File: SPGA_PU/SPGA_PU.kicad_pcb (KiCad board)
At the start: 2 copper layers, 16 parts, among them Q3 NMOS

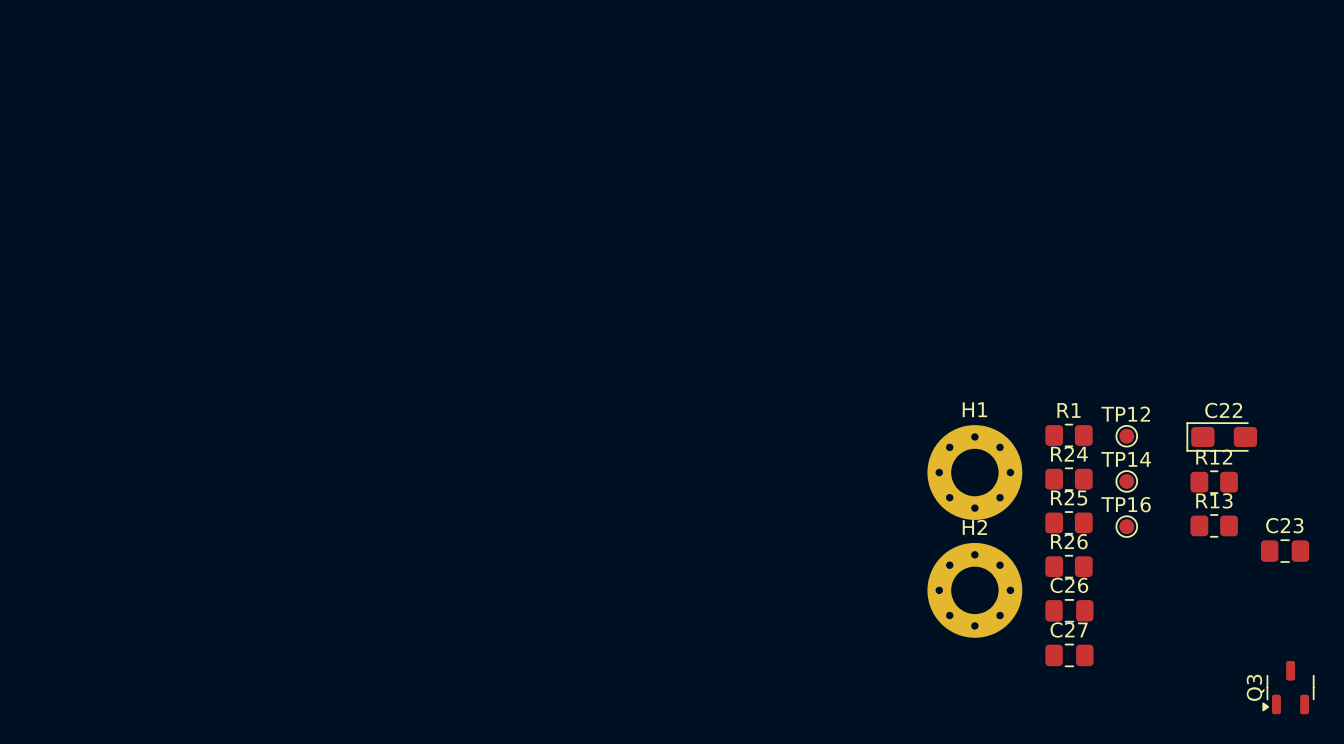
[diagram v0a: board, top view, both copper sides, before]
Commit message: I dunno
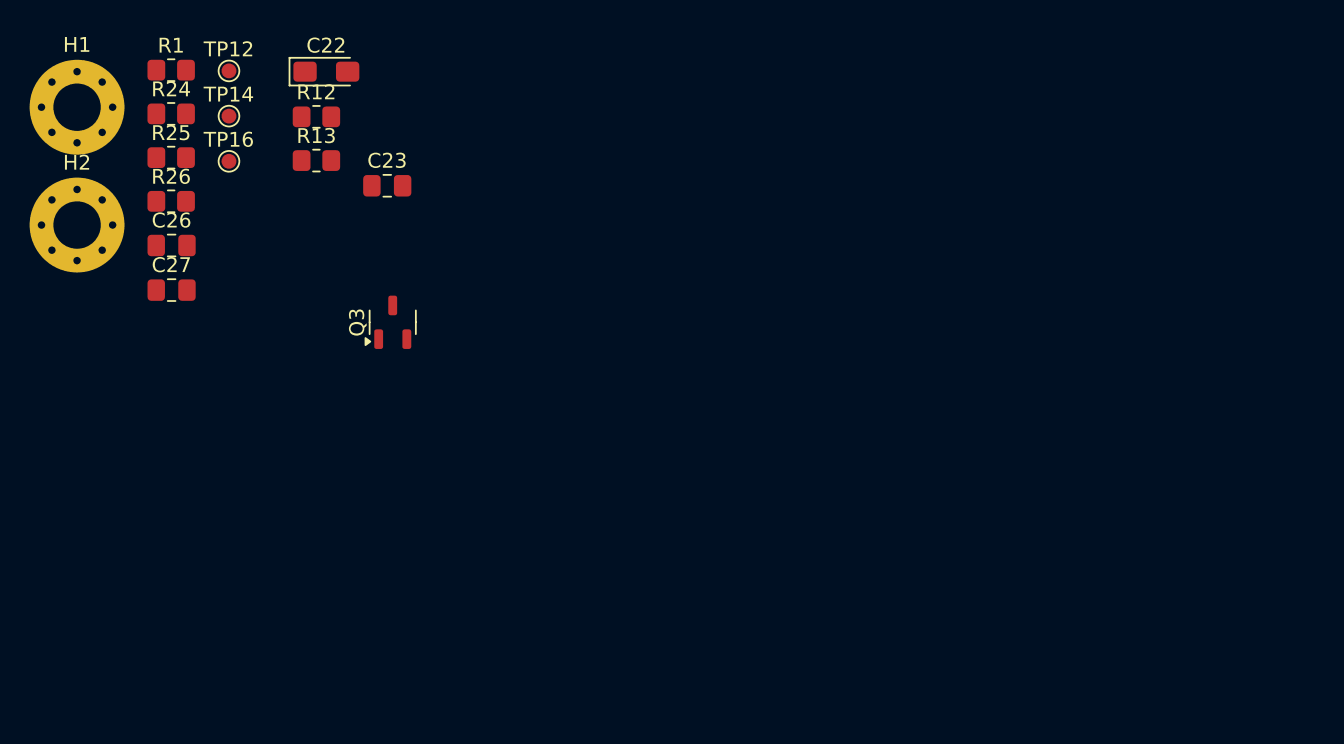
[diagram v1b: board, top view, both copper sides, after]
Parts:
- moved H1 65.4 mm to (38.6, 33.5)
- moved H2 65.4 mm to (38.6, 41.4)
- moved Q3 65.4 mm to (59.9, 48.0)
- moved TP12 65.4 mm to (48.8, 31.0)
- moved TP14 65.4 mm to (48.8, 34.0)
- moved TP16 65.4 mm to (48.8, 37.1)
- moved C22 65.4 mm to (55.4, 31.1)
- moved C23 65.4 mm to (59.5, 38.8)
- moved C26 65.4 mm to (45.0, 42.8)
- moved C27 65.4 mm to (45.0, 45.8)
- moved R1 65.4 mm to (44.9, 30.9)
- moved R12 65.4 mm to (54.7, 34.1)
- moved R13 65.4 mm to (54.7, 37.0)
- moved R24 65.4 mm to (44.9, 33.9)
- moved R25 65.4 mm to (44.9, 36.9)
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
